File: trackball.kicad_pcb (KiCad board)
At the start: 6 copper layers, 65 x 85 mm, 241 parts, among them J2 ZX-PM2.0-2-4PY, Q1 XR2302, Q2 XR2302, SW1 HX TC-5608-Y, SW2 HX TC-5608-Y, SW3 HX TC-5608-Y, SW4 HX TC-5608-Y, SW5 HX TC-5608-Y, SW6 HX TC-5608-Y, SW7 HX TC-5608-Y, SW8 HX TC-5608-Y, SW9 TS-1010-C-A, U1 USB-TYPE-C-017, U10 WS2812B, U11 WS2812B, U12 WS2812B, U13 WS2812B, U14 WS2812B, U15 WS2812B, U16 WS2812B, U17 WS2812B, U18 WS2812B, U19 WS2812B, U2 SY80004DQD, U20 WS2812B, U21 WS2812B, U3 SY80004DQD, U4 PMW3610, U5 PMW3610, U6 WS2812B, U7 WS2812B, U8 WS2812B, U9 WS2812B, X1 XL7EL89CKI-111YLC-32M

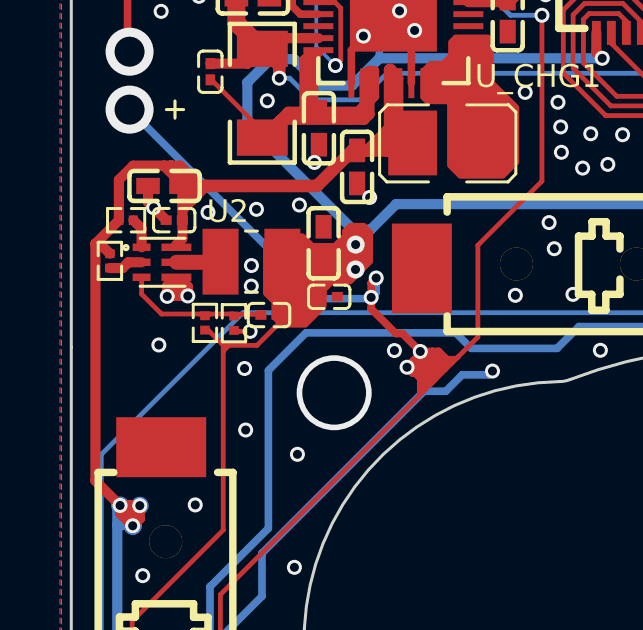
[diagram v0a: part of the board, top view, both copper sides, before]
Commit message: bugfix: 3d models
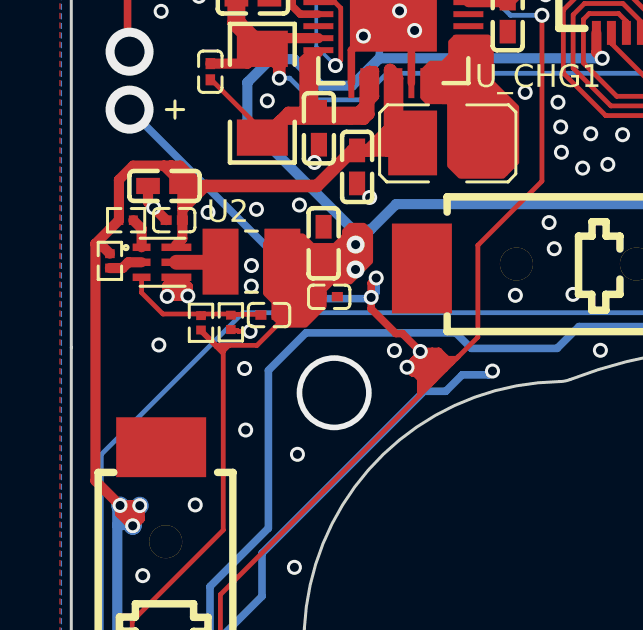
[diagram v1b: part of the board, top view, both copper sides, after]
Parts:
- moved R5 0.13 mm to (36.7, 60.6)
- moved R24 0.11 mm to (37.7, 60.6)
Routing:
- net 1V8: track 307.1 -> 308.7 mm
